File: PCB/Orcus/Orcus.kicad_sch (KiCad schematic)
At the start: 84 parts, among them J1 -, J2 -, J3 +, J4 +, J5 LED, J6 LED, SW1 MX_LED, SW10 MX_LED, SW11 MX_LED, SW12 MX_LED, SW13 MX_LED, SW14 MX_LED, SW15 MX_LED, SW16 MX_LED, SW17 MX_LED, SW18 MX_LED, SW19 MX_LED, SW2 MX_LED, SW20 MX_LED, SW21 MX_LED, SW22 MX_LED, SW23 MX_LED, SW24 MX_LED, SW25 MX_LED, SW26 MX_LED, SW27 MX_LED, SW28 MX_LED, SW29 MX_LED, SW3 MX_LED, SW30 MX_LED, SW31 MX_LED, SW32 MX_LED, SW33 MX_LED, SW34 MX_LED, SW35 MX_LED, SW36 MX_LED, SW37 MX_LED, SW38 MX_LED, SW4 MX_LED, SW5 MX_LED, SW6 MX_LED, SW7 MX_LED, SW8 MX_LED, SW9 MX_LED, U1 XIAO-nRF52840-SMD, U3 XIAO-nRF52840-SMD

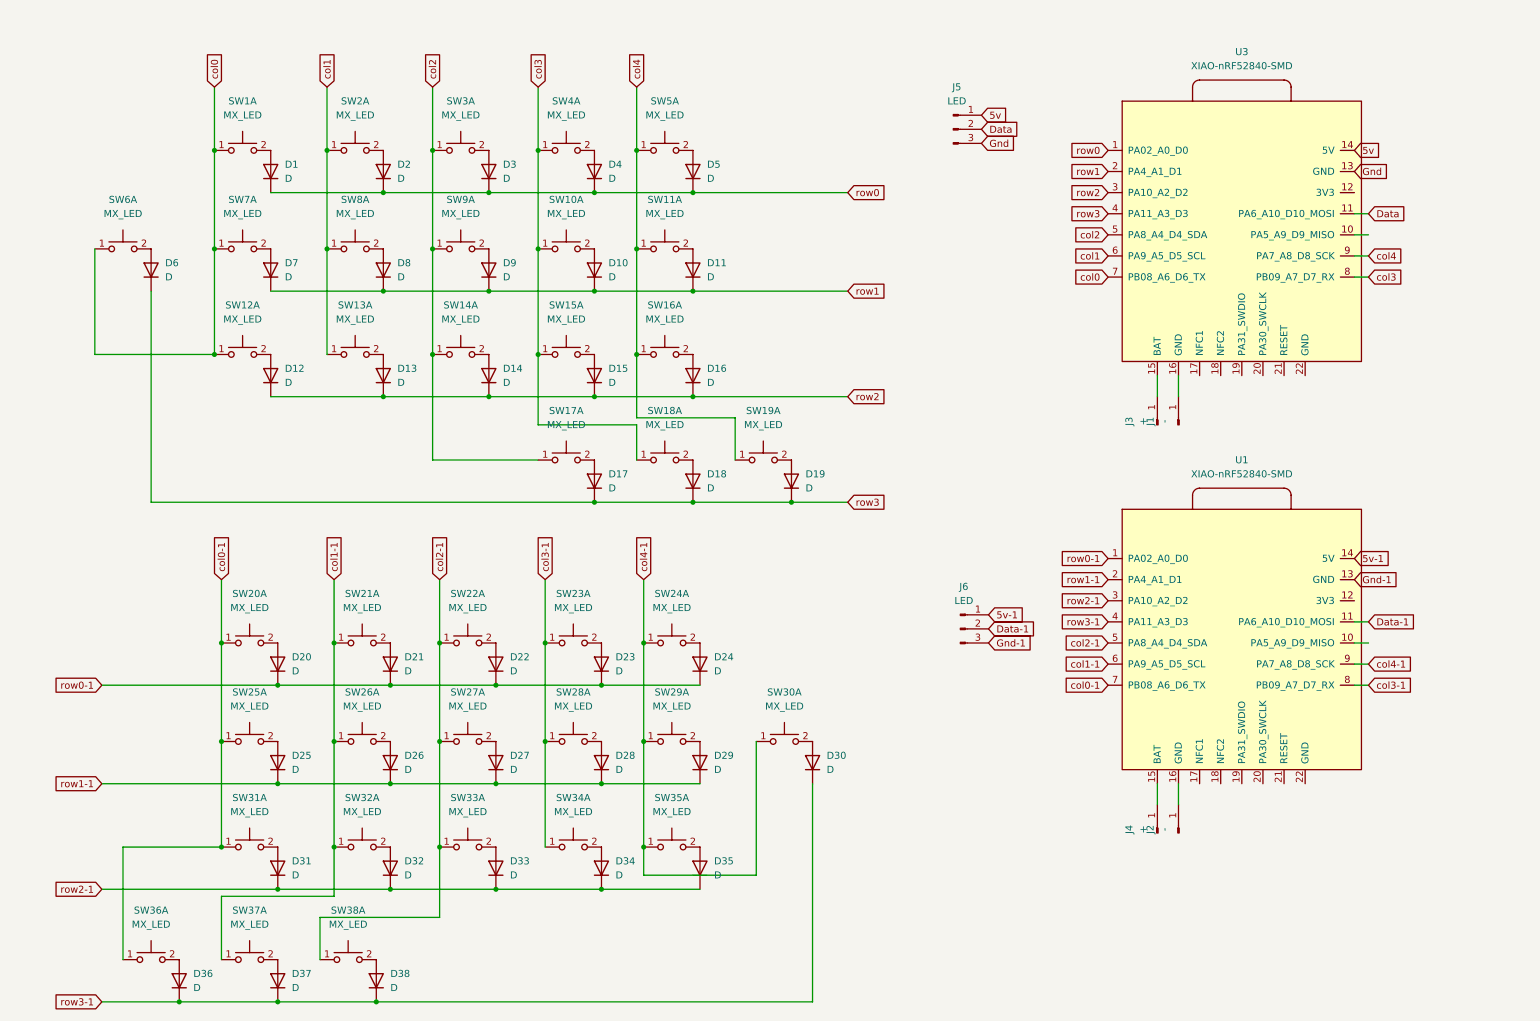
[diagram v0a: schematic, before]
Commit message: new sch
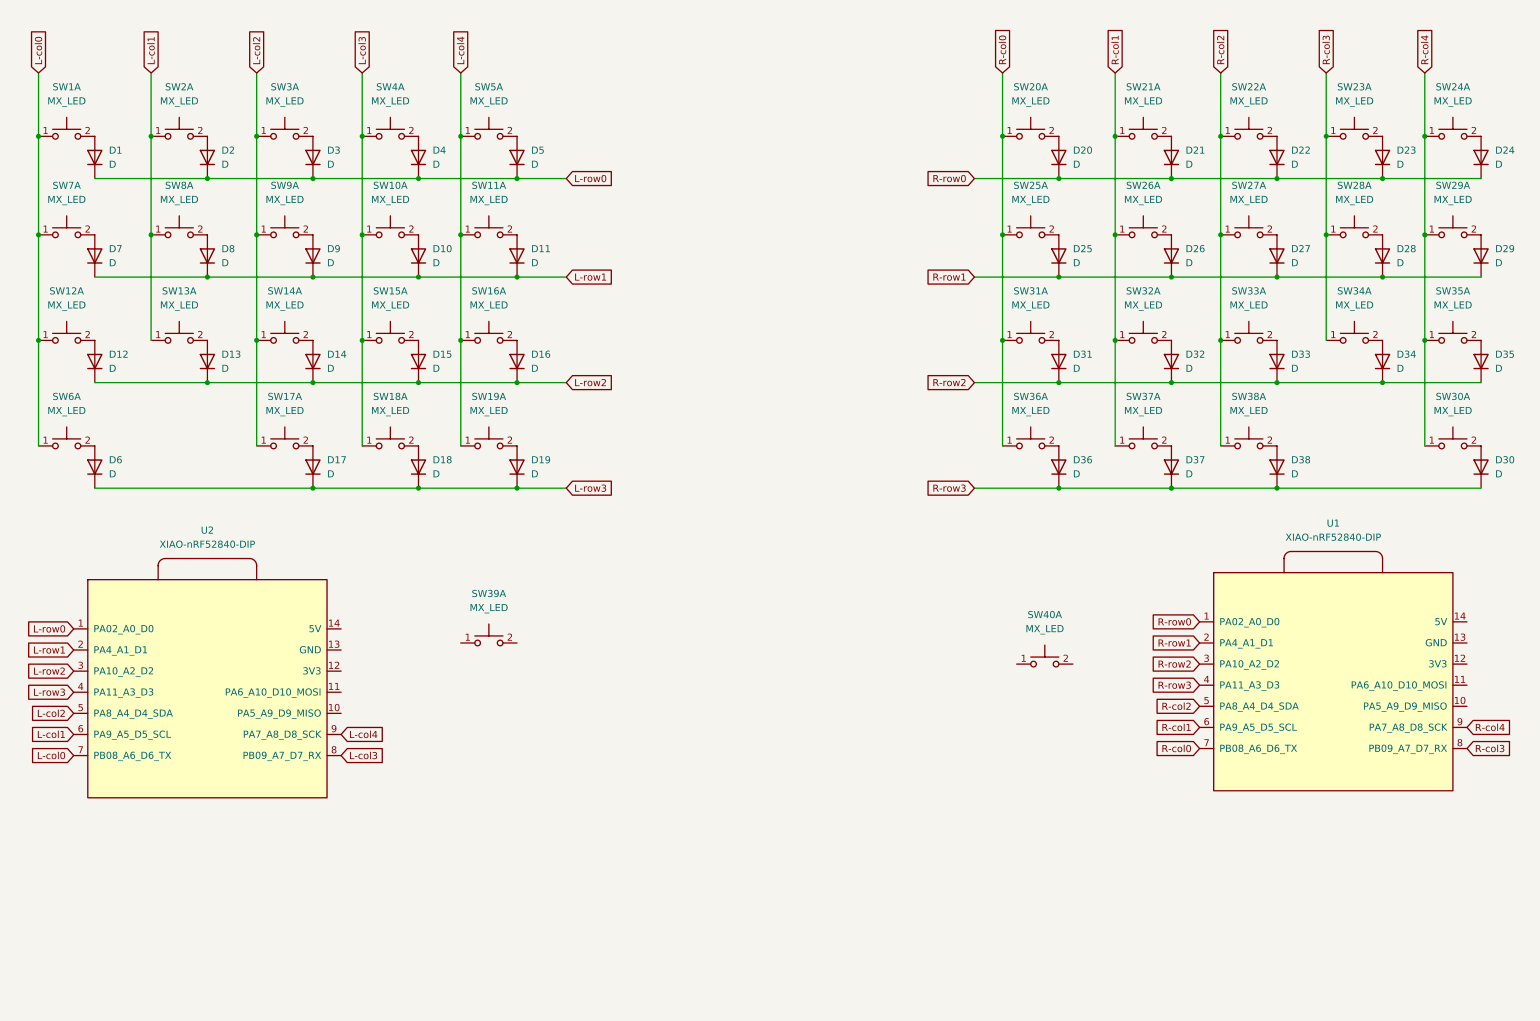
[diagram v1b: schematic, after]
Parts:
- removed J1, J2: -, Keebio-Parts.pretty-master:Wire_Pad_24AWG, symbol Connector:Conn_01x01_Pin
- removed J3, J4: +, Keebio-Parts.pretty-master:Wire_Pad_24AWG, symbol Connector:Conn_01x01_Pin
- removed J5, J6: LED, Keebio-Parts.pretty-master:NeoPixel_Mini_Button-v2, symbol Connector:Conn_01x03_Pin
- removed U1, U3: XIAO-nRF52840-SMD, TOTEMlib:xiao-ble-smd-cutout-mod, symbol MCU_SEEED_XIAO_Series:XIAO-nRF52840-SMD
- added SW39, SW40: MX_LED, Keebio-Parts.pretty-master:Kailh-PG1350-1u-NoLED, symbol keebio:MX_LED
- added U1, U2: XIAO-nRF52840-DIP, MCU_SEEED_XIAO_Series:XIAO-nRF52840-DIP, symbol MCU_SEEED_XIAO_Series:XIAO-nRF52840-DIP
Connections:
- net col0 renamed L-col0
- net L-col0: now also U2.7 (PB08_A6_D6_TX)
- net col0-1 renamed R-col0
- net R-col0: now also U1.7 (PB08_A6_D6_TX)
- net col1 renamed L-col1
- net L-col1: now also U2.6 (PA9_A5_D5_SCL)
- net col1-1 renamed R-col1
- net R-col1: now also U1.6 (PA9_A5_D5_SCL)
- net col2 renamed L-col2
- net L-col2: now also U2.5 (PA8_A4_D4_SDA)
- net col2-1 renamed R-col2
- net R-col2: now also U1.5 (PA8_A4_D4_SDA)
- net col3 renamed L-col3
- net L-col3: now also U2.8 (PB09_A7_D7_RX)
- net col3-1 renamed R-col3
- net R-col3: now also U1.8 (PB09_A7_D7_RX)
- net col4 renamed L-col4
- net L-col4: now also U2.9 (PA7_A8_D8_SCK)
- net col4-1 renamed R-col4
- net R-col4: now also U1.9 (PA7_A8_D8_SCK)
- net row0 renamed L-row0
- net L-row0: now also U2.1 (PA02_A0_D0)
- net row0-1 renamed R-row0
- net R-row0: now also U1.1 (PA02_A0_D0)
- net row1 renamed L-row1
- net L-row1: now also U2.2 (PA4_A1_D1)
- net row1-1 renamed R-row1
- net R-row1: now also U1.2 (PA4_A1_D1)
- net row2 renamed L-row2
- net L-row2: now also U2.3 (PA10_A2_D2)
- net row2-1 renamed R-row2
- net R-row2: now also U1.3 (PA10_A2_D2)
- net row3 renamed L-row3
- net L-row3: now also U2.4 (PA11_A3_D3)
- net row3-1 renamed R-row3
- net R-row3: now also U1.4 (PA11_A3_D3)
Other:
- moved on the sheet: D1, D10, D11, D12, D13, D14, D15, D16, D17, D18, D19, D2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
